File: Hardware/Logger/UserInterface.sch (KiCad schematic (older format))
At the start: 21 parts, among them SW1 SW_Push, SW2 SW_Push, SW3 SW_Push, SW4 SW_Push, U2 ST7735S

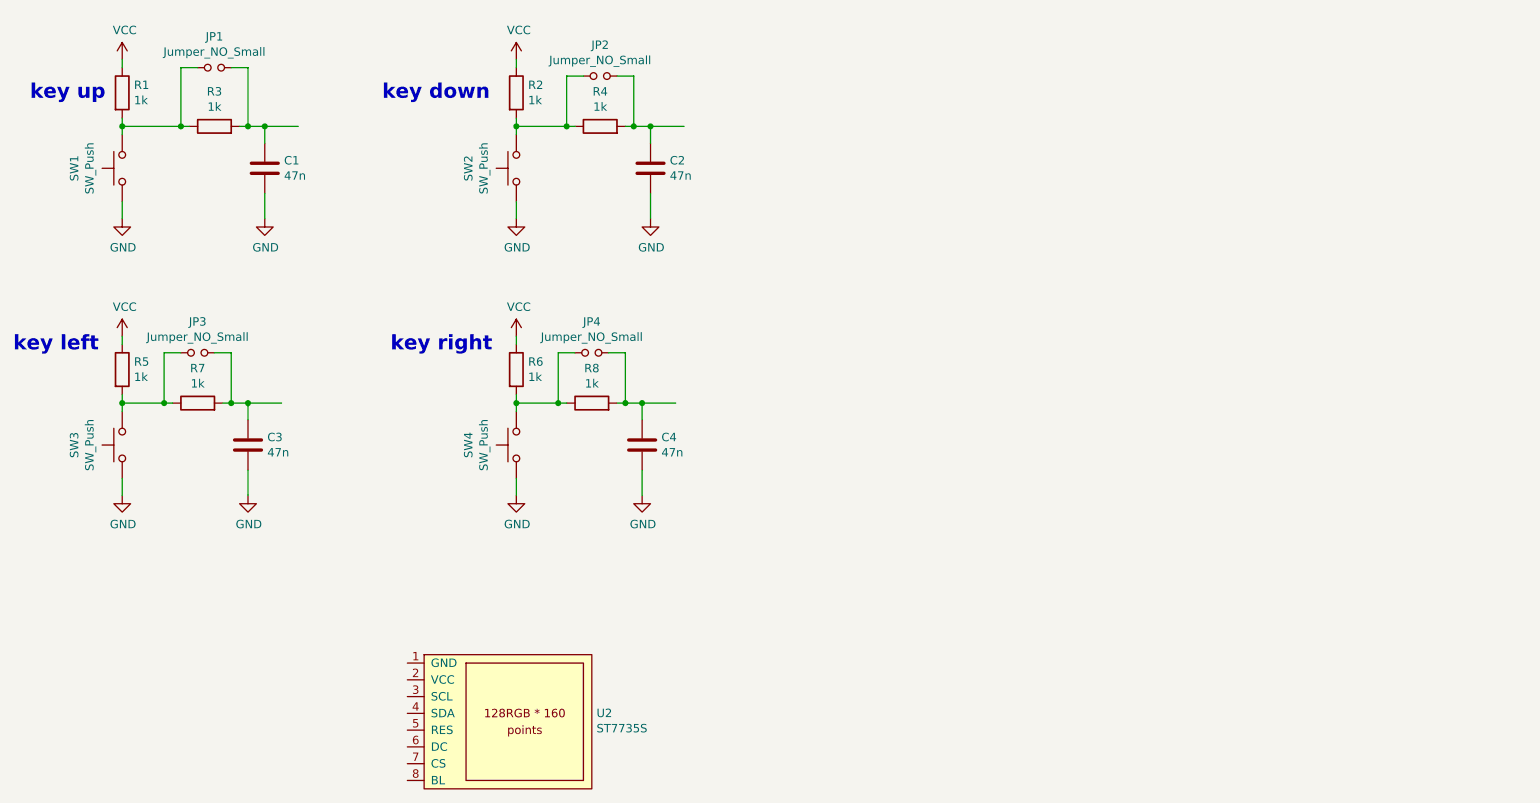
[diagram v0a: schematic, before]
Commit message: fix #27, fix #30, fix #32
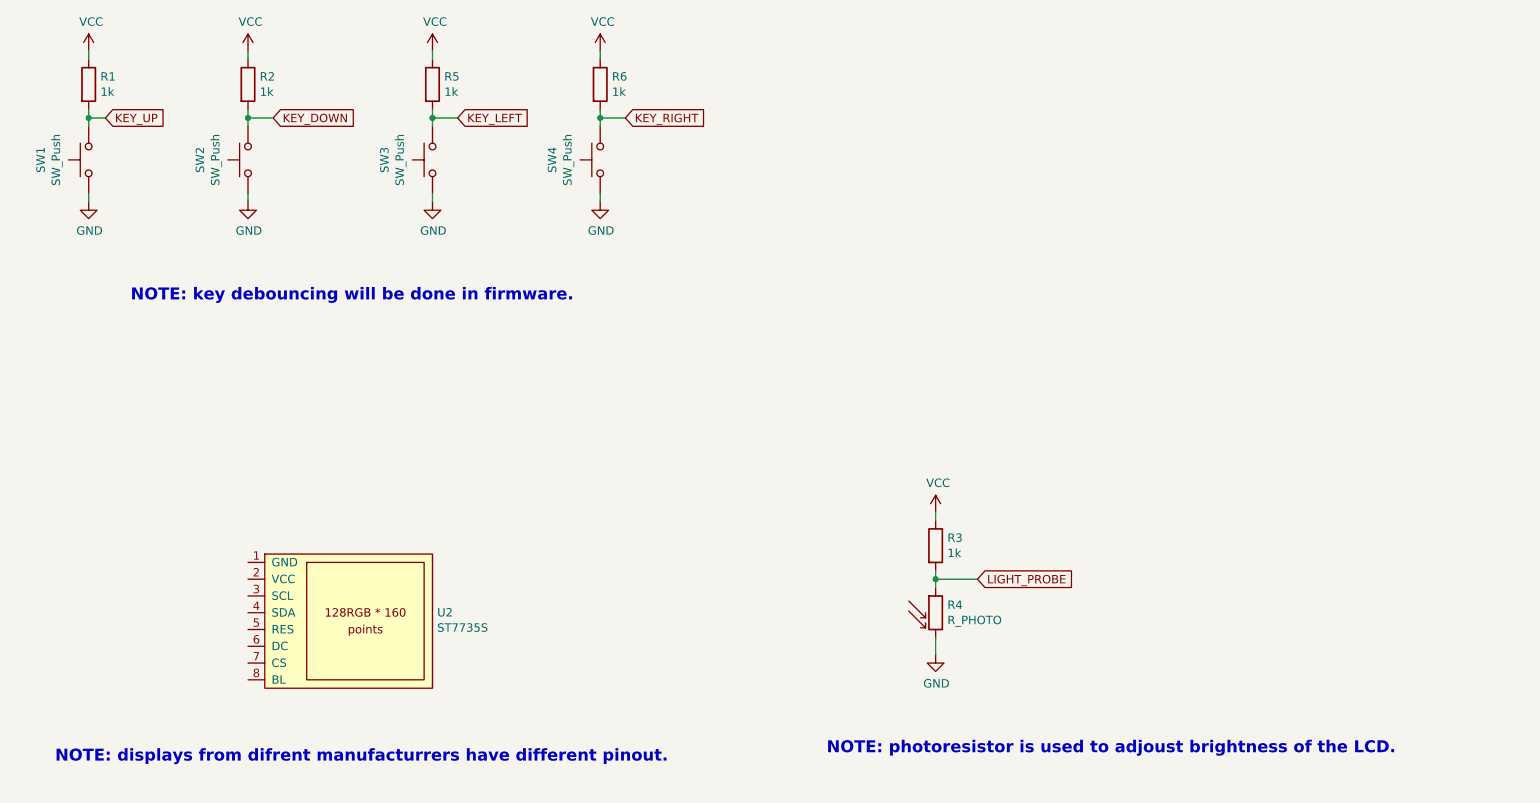
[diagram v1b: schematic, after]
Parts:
- removed C1, C2, C3, C4: 47n, Capacitor_SMD:C_0805_2012Metric, symbol Device:C
- removed JP1, JP2, JP3, JP4: Jumper_NO_Small, Jumper:SolderJumper-2_P1.3mm_Open_Pad1.0x1.5mm, symbol Device:Jumper_NO_Small
- removed R4, R7, R8: 1k, Resistor_SMD:R_0805_2012Metric, symbol Device:R
- added R4: R_PHOTO, OptoDevice:R_LDR_7x6mm_P5.1mm_Vertical, symbol Device:R_PHOTO
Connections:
- net labels added: KEY_DOWN, KEY_LEFT, KEY_RIGHT, KEY_UP, LIGHT_PROBE
- wire segments 60 -> 25
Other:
- note added: "NOTE: displays from difrent manufacturrers have different pinout."
- note added: "NOTE: key debouncing will be done in firmware."
- note added: "NOTE: photoresistor is used to adjoust brightness of the LCD."
- note removed: "key down"
- note removed: "key left"
- note removed: "key right"
- note removed: "key up"
- moved on the sheet: R1, R2, R5, R6, SW1, SW2, SW3, SW4, U2
